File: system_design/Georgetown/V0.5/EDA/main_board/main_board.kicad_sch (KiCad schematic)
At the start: 31 parts, among them J1 B3B-XH-A_LF__SN_, J2 Conn_01x02_Pin, P1 SD card socket, U1 HX-2S-JH10, U2 DS3231M, U3 INA219AxD, U4 BME280_module, U5 KA78M05_TO252

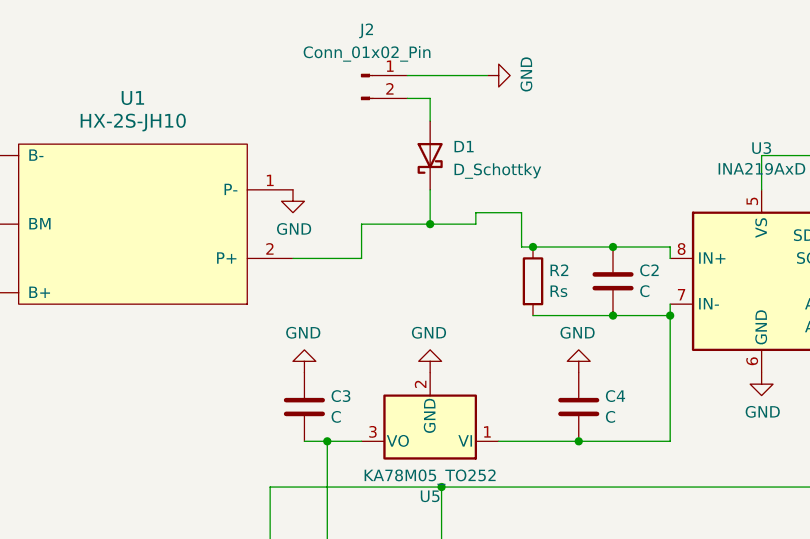
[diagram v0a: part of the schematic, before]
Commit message: PCB design modified
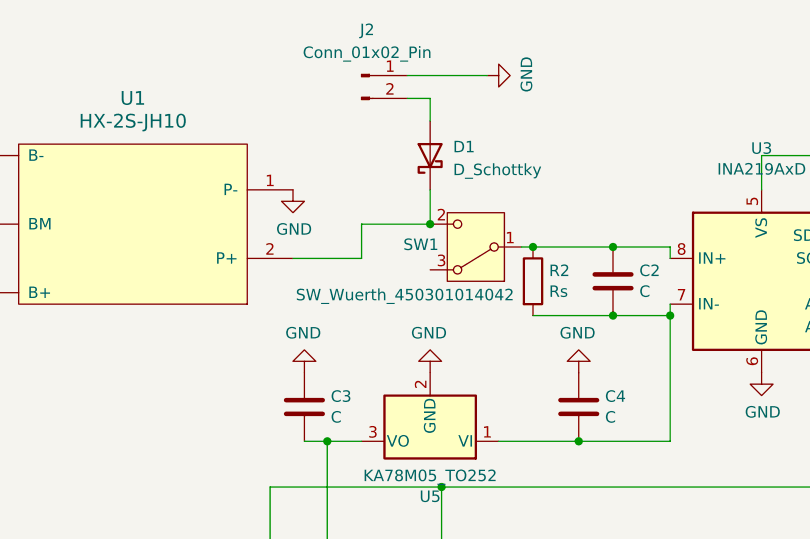
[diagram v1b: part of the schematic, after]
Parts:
- added SW1: SW_Wuerth_450301014042, Button_Switch_THT:SW_Slide-03_Wuerth-WS-SLTV_10x2.5x6.4_P2.54mm, symbol Switch:SW_Wuerth_450301014042
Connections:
- net at C2.1, R2.1, U3.8 (IN+): now also SW1.1 (B); no longer D1.1 (K), U1.2 (P+)
- new net: D1.1 (K), SW1.2 (C), U1.2 (P+)
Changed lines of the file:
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@@
 	(wire
 		(pts
-			(xy 95.25 34.29) (xy 95.25 38.1)
-		)
-		(stroke
-			(width 0)
-			(type default)
-		)
-	)
-	(wire
-		(pts
 			(xy 132.08 144.78) (xy 135.89 144.78)
 		)
@@
 	(wire
 		(pts
-			(xy 85.09 35.56) (xy 90.17 35.56)
-		)
-		(stroke
-			(width 0)
-			(type default)
-		)
-	)
-	(wire
-		(pts
 			(xy 101.6 115.57) (xy 162.56 115.57)
 		)
@@
 	(wire
 		(pts
-			(xy 90.17 35.56) (xy 90.17 34.29)
-		)
-		(stroke
-			(width 0)
-			(type default)
-		)
-	)
-	(wire
-		(pts
 			(xy 86.36 152.4) (xy 86.36 156.21)
 		)
@@
 	(wire
 		(pts
-			(xy 90.17 34.29) (xy 95.25 34.29)
-		)
-		(stroke
-			(width 0)
-			(type default)
-		)
-	)
-	(wire
-		(pts
 			(xy 101.6 59.69) (xy 111.76 59.69)
 		)
@@
 					(unit 1)
 				)
+			)
+		)
+	)
+	(symbol
+		(lib_id "Switch:SW_Wuerth_450301014042")
+		(at 90.17 38.1 180)
+		(unit 1)
+		(exclude_from_sim no)
+		(in_bom yes)
+		(on_board yes)
+		(dnp no)
+		(property "Reference" "SW1"
+			(at 84.074 37.846 0)
+			(effects
+				(font
+					(size 1.27 1.27)
+				)
+			)
+		)
+		(property "Value" "SW_Wuerth_450301014042"
+			(at 82.296 43.434 0)
+			(effects
+				(font
+					(size 1.27 1.27)
+				)
+			)
+		)
+		(property "Footprint" "Button_Switch_THT:SW_Slide-03_Wuerth-WS-SLTV_10x2.5x6.4_P2.54mm"
+			(at 90.17 27.94 0)
+			(effects
+				(font
+					(size 1.27 1.27)
+				)
+				(hide yes)
+			)
+		)
+		(property "Datasheet" "https://www.we-online.com/components/products/datasheet/450301014042.pdf"
+			(at 90.17 30.48 0)
+			(effects
+				(font
+					(size 1.27 1.27)
+				)
+				(hide yes)
+			)
+		)
+		(property "Description" "Switch slide, single pole double throw"
+			(at 90.17 38.1 0)
+			(effects
+				(font
+					(size 1.27 1.27)
+				)
+				(hide yes)
+			)
+		)
+		(pin "3"
+		)
+		(pin "1"
+		)
+		(pin "2"
+		)
+		(instances
+			(project ""
+				(path "/6055025c-91fc-4d42-99c1-24bcdc7ae09f"
+					(reference "SW1")
+					(unit 1)
+				)
